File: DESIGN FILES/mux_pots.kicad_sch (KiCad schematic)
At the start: 20 parts, among them U701 CD74HC4067, U702 ENCODER

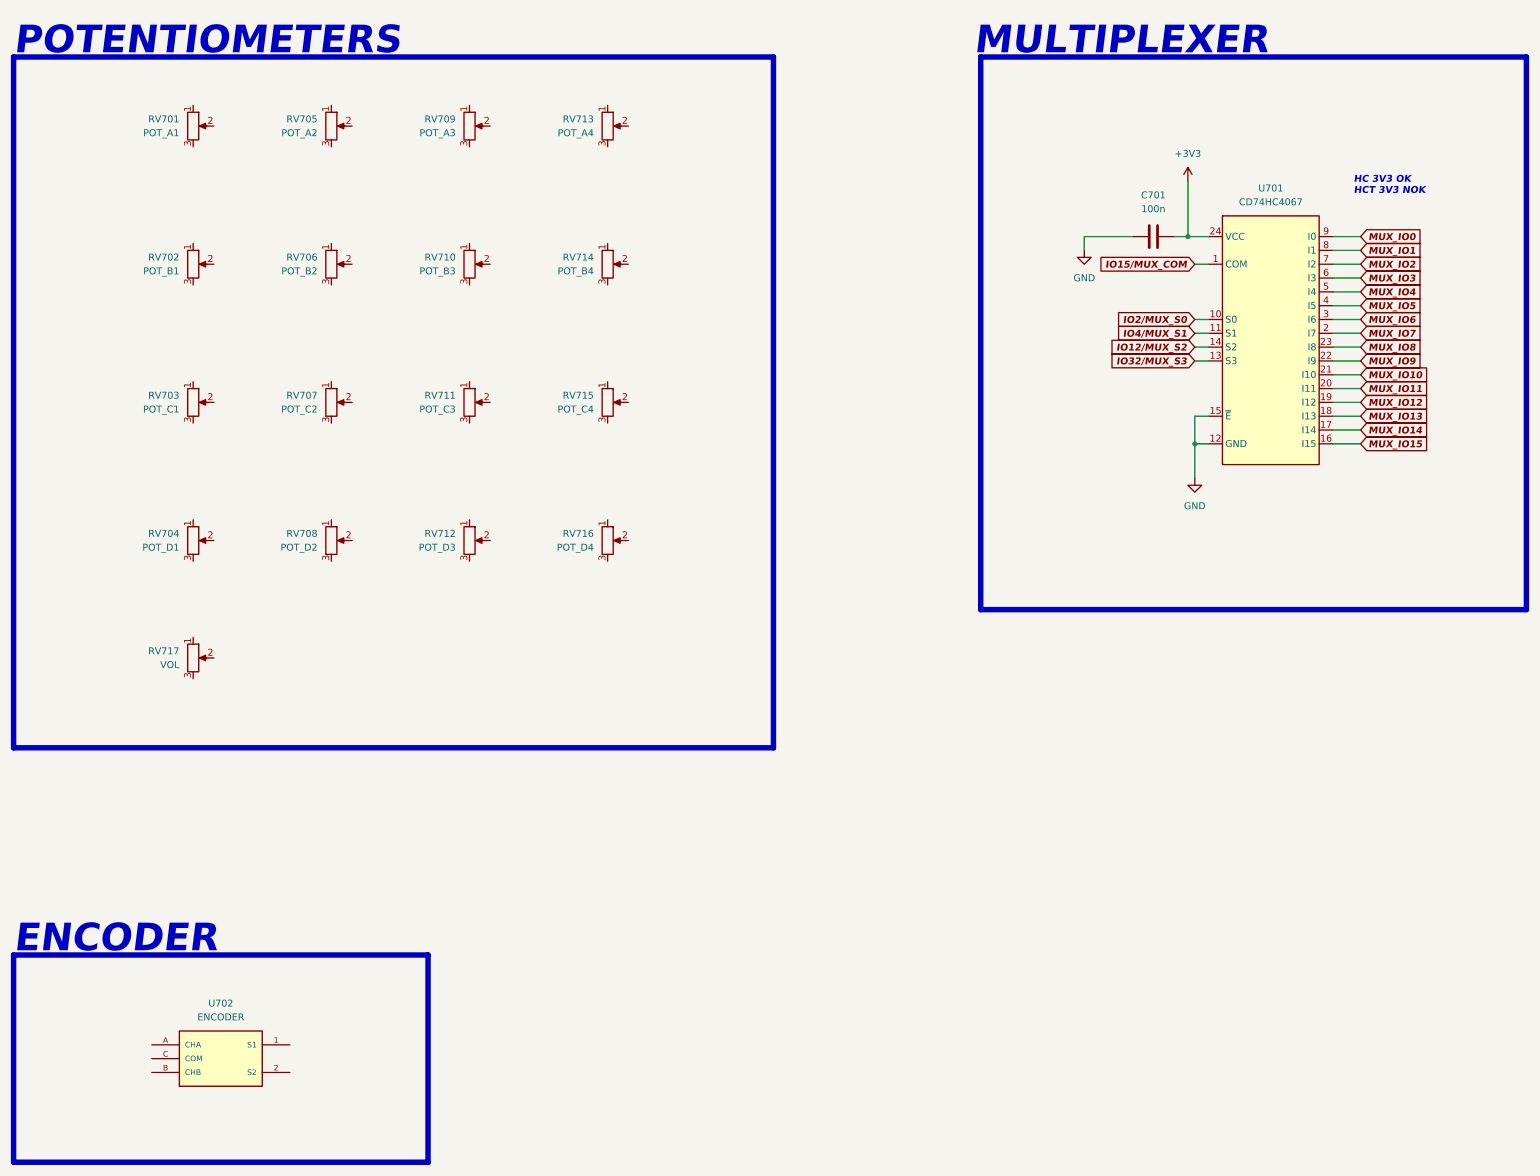
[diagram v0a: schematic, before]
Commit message: updates
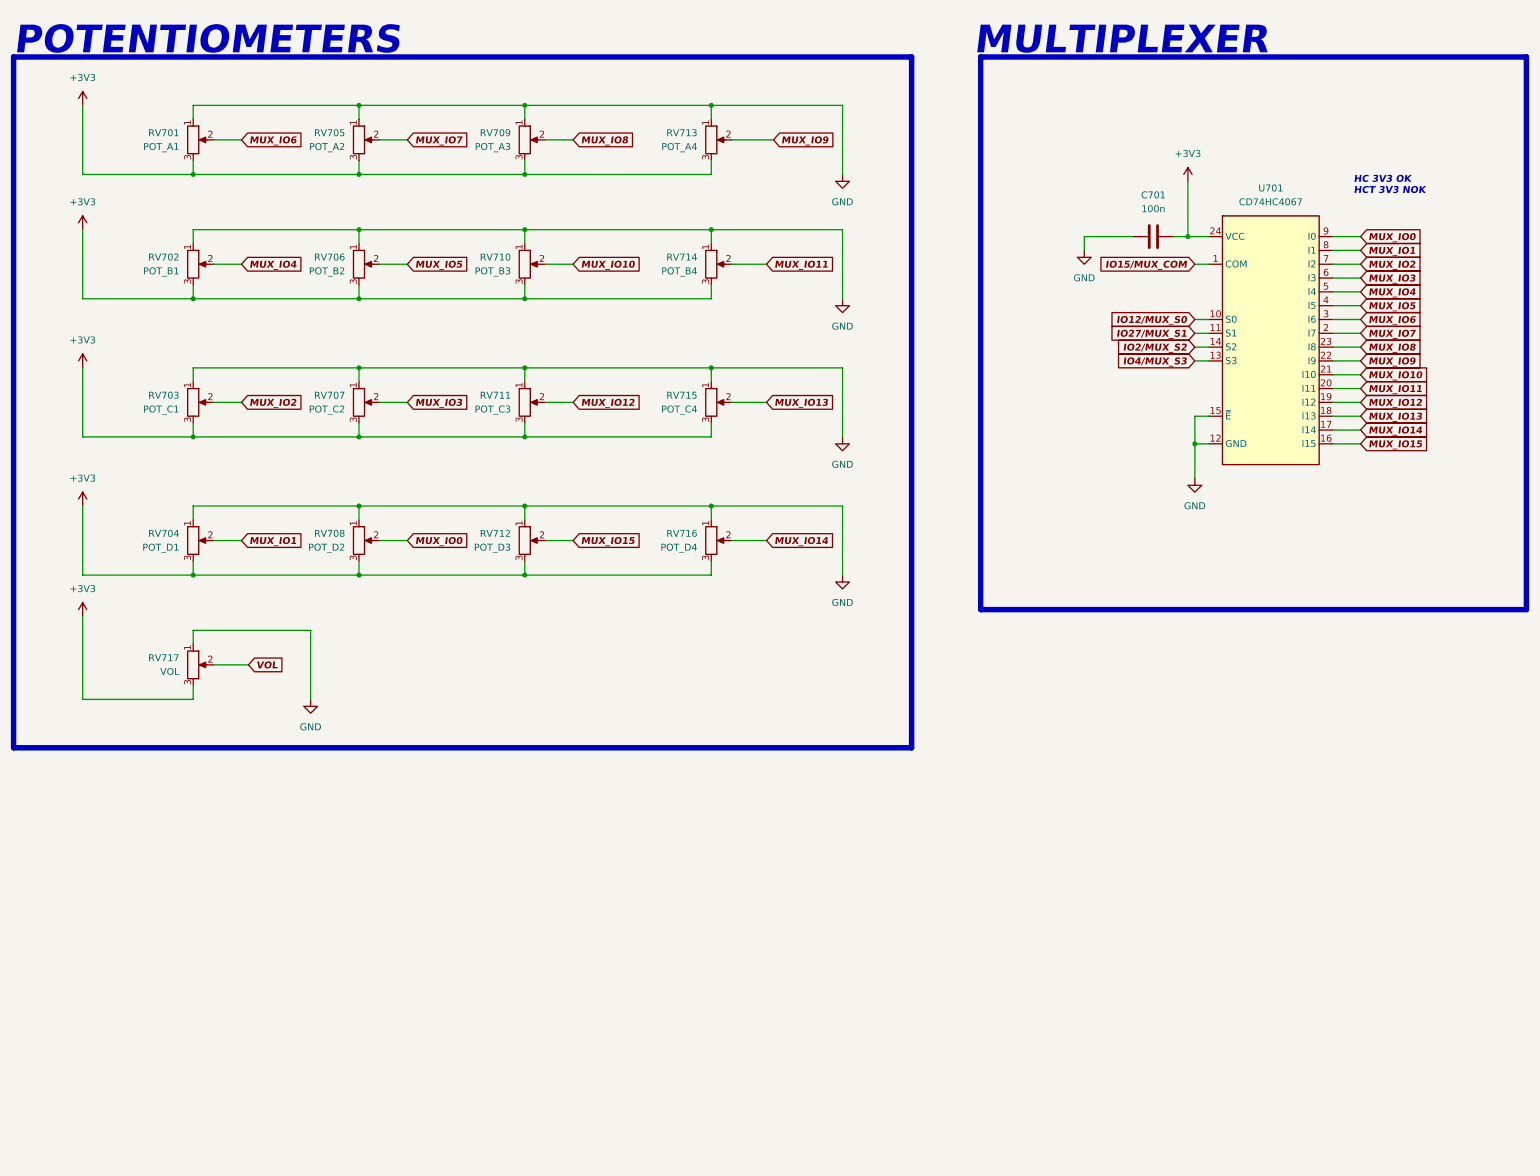
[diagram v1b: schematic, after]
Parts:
- removed U702: ENCODER, MY ENCODER LIBRARY:ENC_PEC12R-4025F-S0024, symbol MY ENCODER LIBRARY:PEC12R-4025F-S0024
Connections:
- net +3V3: now also RV701.3, RV702.3, RV703.3, RV704.3, RV705.3, RV706.3, RV707.3, RV708.3, RV709.3, RV710.3, RV711.3, RV712.3, RV713.3, RV714.3, RV715.3, RV716.3, RV717.3
- net GND: now also RV701.1, RV702.1, RV703.1, RV704.1, RV705.1, RV706.1, RV707.1, RV708.1, RV709.1, RV710.1, RV711.1, RV712.1, RV713.1, RV714.1, RV715.1, RV716.1, RV717.1
- net MUX_IO0: now also RV708.2
- net MUX_IO1: now also RV704.2
- net MUX_IO10: now also RV710.2
- net MUX_IO11: now also RV714.2
- net MUX_IO12: now also RV711.2
- net MUX_IO13: now also RV715.2
- net MUX_IO14: now also RV716.2
- net MUX_IO15: now also RV712.2
- net MUX_IO2: now also RV703.2
- net MUX_IO3: now also RV707.2
- net MUX_IO4: now also RV702.2
- net MUX_IO5: now also RV706.2
- net MUX_IO6: now also RV701.2
- net MUX_IO7: now also RV705.2
- net MUX_IO8: now also RV709.2
- net MUX_IO9: now also RV713.2
- net VOL: now reaches RV717.2
- net IO12/MUX_S2 renamed IO2/MUX_S2
- net IO2/MUX_S0 renamed IO12/MUX_S0
- net IO32/MUX_S3 renamed IO4/MUX_S3
- net IO4/MUX_S1 renamed IO27/MUX_S1
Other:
- note removed: "ENCODER"
- moved on the sheet: RV701, RV705, RV706, RV707, RV708, RV709, RV710, RV711, RV712, RV713, RV714, RV715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
